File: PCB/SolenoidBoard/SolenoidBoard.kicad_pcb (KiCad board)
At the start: 2 copper layers, 90 x 60 mm, 21 parts, among them J1 XT30, J2 Con_45V, J3 Con_45V, J4 Conn_01x02, J5 Con_GND, J6 Con_GND, J7 Conn_01x03, U1 TLP293, U2 TLP293

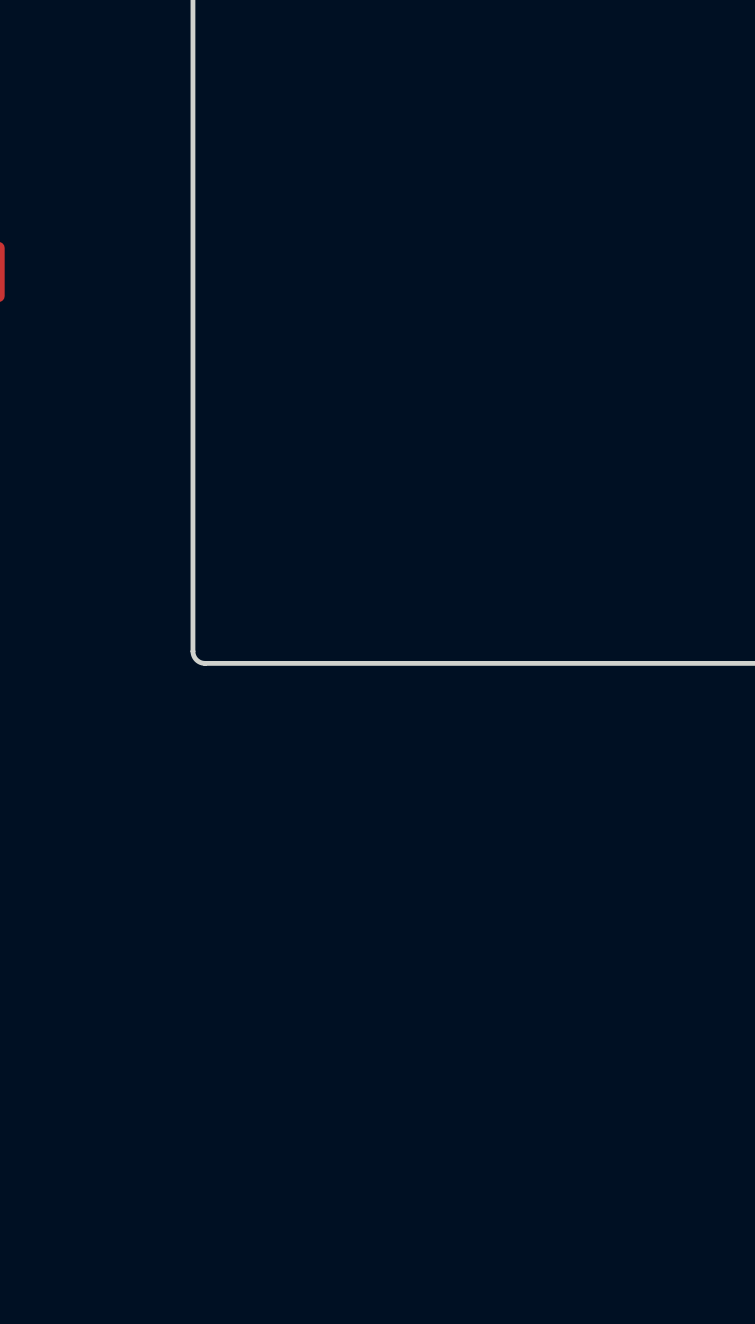
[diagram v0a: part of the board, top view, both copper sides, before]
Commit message: 回路図完成
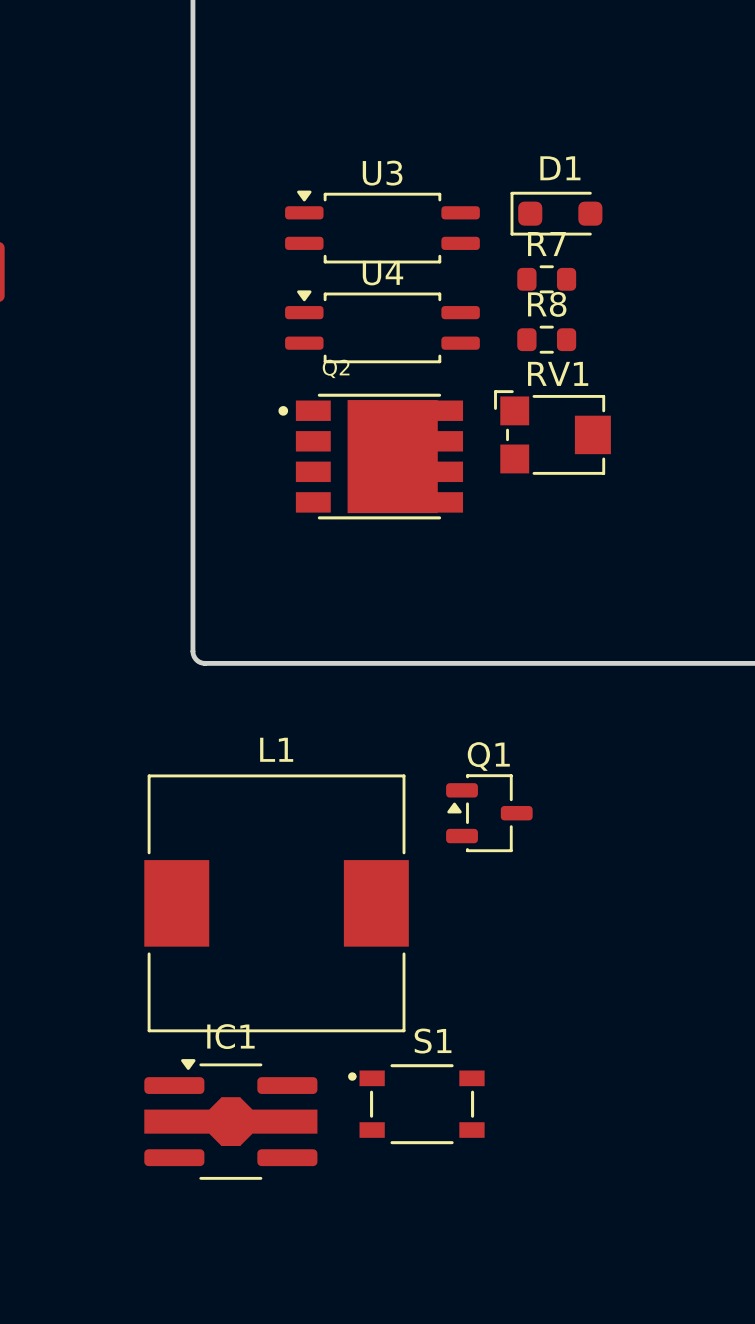
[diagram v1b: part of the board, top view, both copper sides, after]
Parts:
- added D1: CUHS20S60,H3F, Diode_SMD:D_SOD-323_HandSoldering, F.Cu at (169.3, 64.2)
- added IC1: NJW4132U2-B-TE2, Package_TO_SOT_SMD:SOT-89-5_Handsoldering, F.Cu at (155.6, 101.9)
- added L1: NR10050T470M, Inductor_SMD:L_10.4x10.4_H4.8, F.Cu at (157.5, 92.8)
- added Q1: Q_PMOS_GSD, Package_TO_SOT_SMD:SOT-23-3, F.Cu at (166.3, 89.1)
- added Q2: TPH11006NL,LQ_S, SOP Advance:SOP Advance, F.Cu at (161.8, 74.3)
- added R7: 330, Resistor_SMD:R_0603_1608Metric, F.Cu at (168.7, 66.9)
- added R8: 330, Resistor_SMD:R_0603_1608Metric, F.Cu at (168.7, 69.4)
- added RV1: 50k, Potentiometer_SMD:Potentiometer_Bourns_TC33X_Vertical, F.Cu at (169.2, 73.4)
- added S1: SKRPACE010, SKRPACE010:SW_SKRPACE010, F.Cu at (163.5, 101.2)
- added U3: TLP293, Package_SO:SOIC-4_4.55x2.6mm_P1.27mm, F.Cu at (161.9, 64.8)
- added U4: TLP293, Package_SO:SOIC-4_4.55x2.6mm_P1.27mm, F.Cu at (161.9, 68.9)
